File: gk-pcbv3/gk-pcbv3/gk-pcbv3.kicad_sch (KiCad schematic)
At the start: 83 parts, among them J1 USB_C_Receptacle_USB2.0, J10 Barrel_Jack_Switch, J12 Conn_01x02, J2 Conn_01x02, J8 Conn_ARM_JTAG_SWD_10, U1 WE-TVS-82400102, U10 MAX17048, U13 LTC3536xMSE, U15 MAX40203AUK, U16 MAX40203AUK, U2 MCP73831-2-OT, U3 AP62300WU

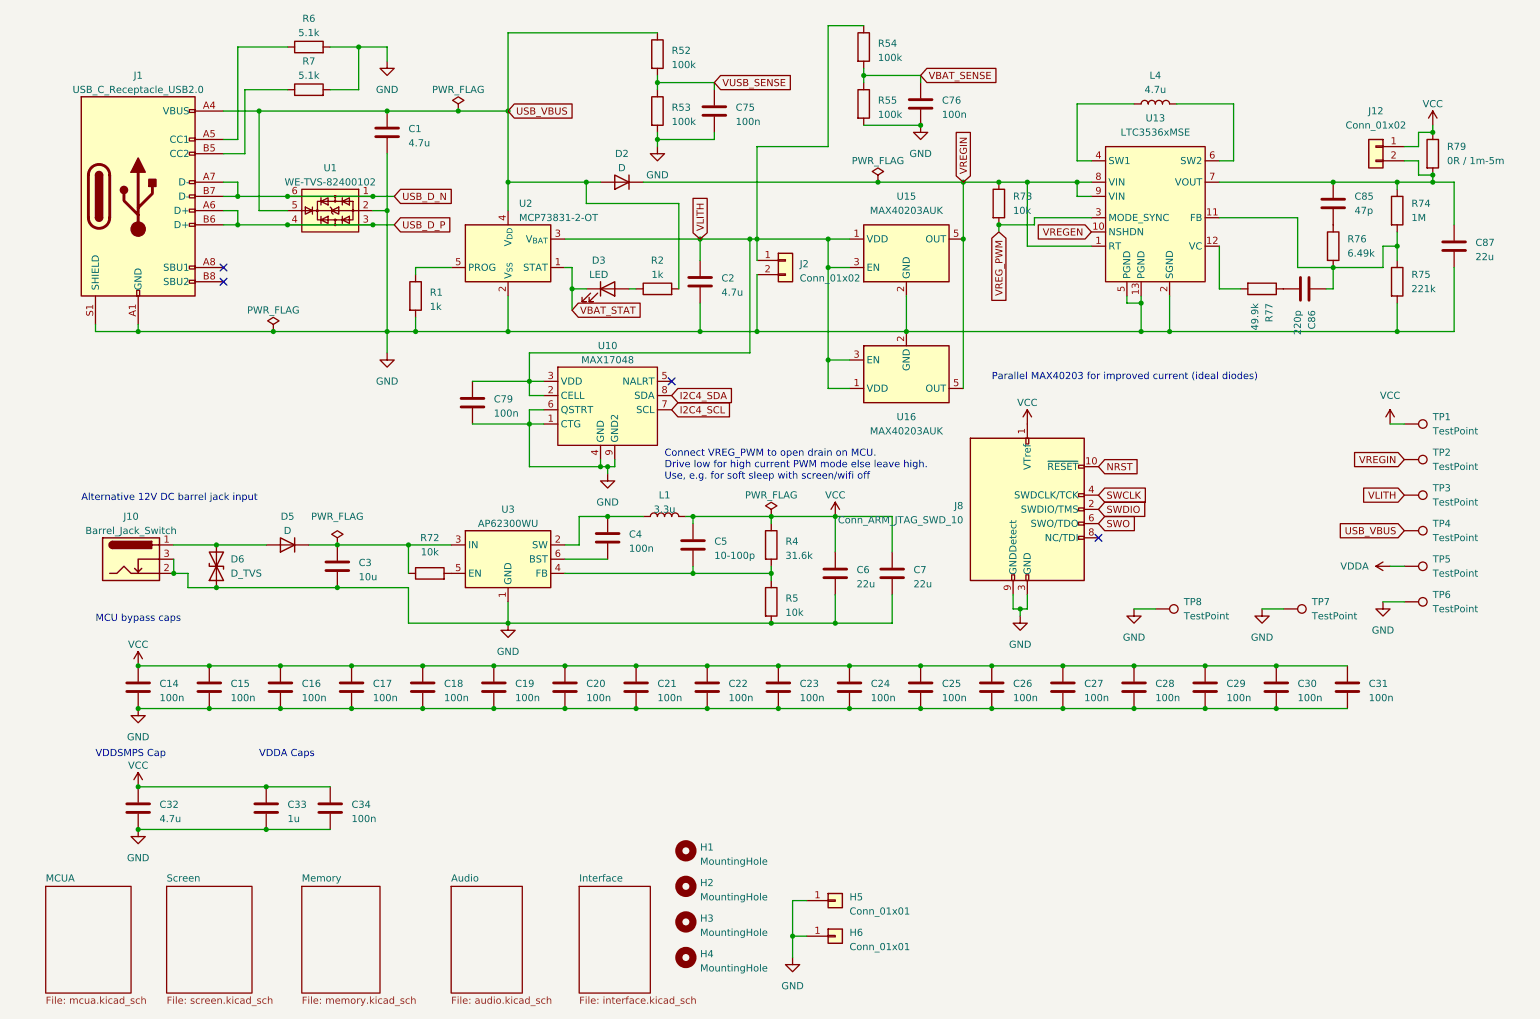
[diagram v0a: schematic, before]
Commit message: v3 board
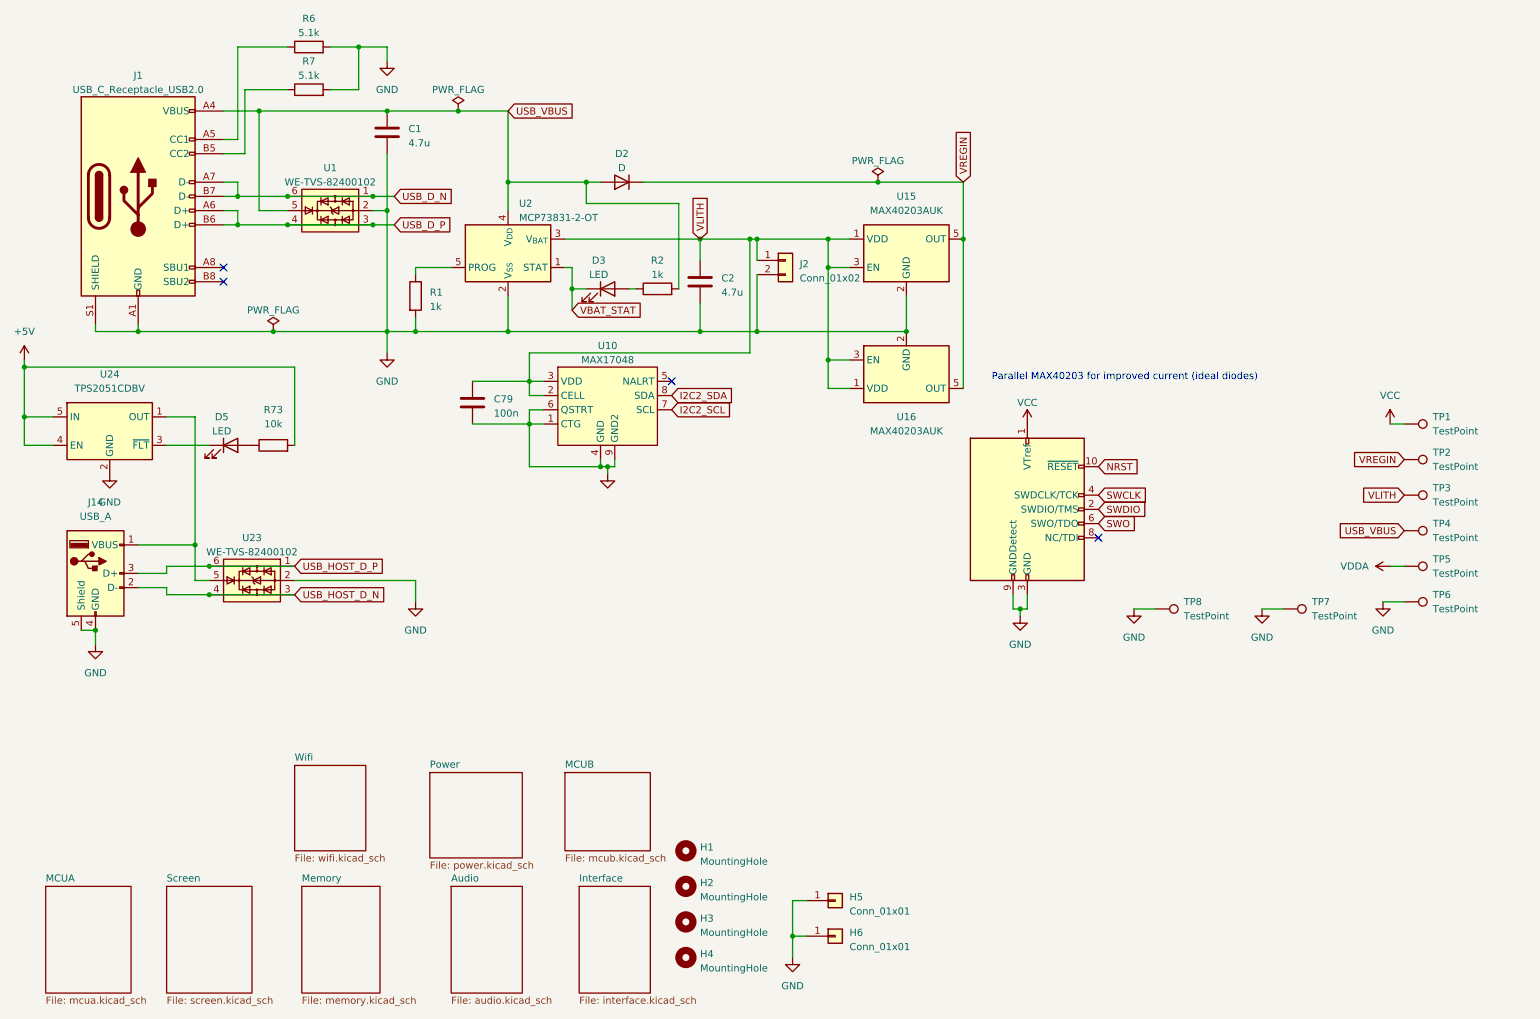
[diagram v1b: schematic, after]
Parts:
- removed C14, C15, C16, C17, C18, C19, C20, C21, C22, C23, C24, C25, C26, C27, C28, C29, C30, C31, C34, C4, C75, C76: 100n, Capacitor_SMD:C_0603_1608Metric, symbol Device:C
- removed C3: 10u, Capacitor_SMD:C_0805_2012Metric, symbol Device:C
- removed C32: 4.7u, Capacitor_SMD:C_0805_2012Metric, symbol Device:C
- removed C33: 1u, Capacitor_SMD:C_0805_2012Metric, symbol Device:C
- removed C5: 10-100p, Capacitor_SMD:C_0603_1608Metric, symbol Device:C
- removed C6, C7, C87: 22u, Capacitor_SMD:C_0805_2012Metric, symbol Device:C
- removed C85: 47p, Capacitor_SMD:C_0603_1608Metric, symbol Device:C
- removed C86: 220p, Capacitor_SMD:C_0603_1608Metric, symbol Device:C
- removed D5: D, Diode_SMD:D_SOD-128, symbol Device:D
- removed D6: D_TVS, Diode_SMD:D_SMA, symbol Device:D_TVS
- removed J10: Barrel_Jack_Switch, Connector_BarrelJack:BarrelJack_Horizontal, symbol Connector:Barrel_Jack_Switch
- removed J12: Conn_01x02, Connector_PinHeader_2.54mm:PinHeader_1x02_P2.54mm_Vertical, symbol Connector_Generic:Conn_01x02
- removed L1: 3.3u, Inductor_SMD:L_7.3x7.3_H4.5, symbol Device:L
- removed L4: 4.7u, Inductor_SMD:L_7.3x7.3_H4.5, symbol Device:L
- removed R4: 31.6k, Resistor_SMD:R_0603_1608Metric, symbol Device:R
- removed R5, R72: 10k, Resistor_SMD:R_0603_1608Metric, symbol Device:R
- removed R52, R53, R54, R55: 100k, Resistor_SMD:R_0603_1608Metric, symbol Device:R
- removed R74: 1M, Resistor_SMD:R_0603_1608Metric, symbol Device:R
- removed R75: 221k, Resistor_SMD:R_0603_1608Metric, symbol Device:R
- removed R76: 6.49k, Resistor_SMD:R_0603_1608Metric, symbol Device:R
- removed R77: 49.9k, Resistor_SMD:R_0603_1608Metric, symbol Device:R
- removed R79: 0R / 1m-5m, Resistor_SMD:R_2512_6332Metric, symbol Device:R
- removed U13: LTC3536xMSE, Package_SO:MSOP-12-1EP_3x4mm_P0.65mm_EP1.65x2.85mm, symbol gk-syms:LTC3536xMSE
- removed U3: AP62300WU, Package_TO_SOT_SMD:TSOT-23-6, symbol Regulator_Switching:AP62300WU
- added D5: LED, LED_SMD:LED_0603_1608Metric, symbol Device:LED
- added J14: USB_A, Connector_USB:USB_A_Molex_67643_Horizontal, symbol Connector:USB_A
- added U23: WE-TVS-82400102, Package_TO_SOT_SMD:SOT-23-6, symbol Power_Protection:WE-TVS-82400102
- added U24: TPS2051CDBV, Package_TO_SOT_SMD:SOT-23-5, symbol Power_Management:TPS2051CDBV
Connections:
- net GND: now also J14.4 (GND), J14.5 (Shield), U23.2, U24.2 (GND)
- net VREGIN: no longer R73.1
- net I2C4_SCL renamed I2C2_SCL
- net I2C4_SDA renamed I2C2_SDA
- net VREG_PWM renamed +5V
- net +5V: now also U24.4 (EN), U24.5 (IN)
- new net: D5.1 (K), U24.3 (~{FLT})
- new net: D5.2 (A), R73.1
- new net: J14.1 (VBUS), U23.5, U24.1 (OUT)
- new net USB_HOST_D_N: J14.2 (D-), U23.3, U23.4
- new net USB_HOST_D_P: J14.3 (D+), U23.1, U23.6
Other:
- added sheet MCUB (mcub.kicad_sch)
- added sheet Power (power.kicad_sch)
- added sheet Wifi (wifi.kicad_sch)
- note removed: "Alternative 12V DC barrel jack input"
- note removed: "Connect VREG_PWM to open drain on MCU. Drive low for high current PWM mode else leave high. Use, e.g. for soft sleep with screen/wifi off"
- note removed: "MCU bypass caps"
- note removed: "VDDA Caps"
- note removed: "VDDSMPS Cap"
